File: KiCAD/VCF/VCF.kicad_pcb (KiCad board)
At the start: 2 copper layers, 50 x 100 mm, 50 parts, among them J1 FM, J2 CV, J3 IN, J4 OUT, J5 Conn_01x03, J6 Conn_01x03, Q1 2N3904, SW1 SW_SPDT, SW2 SW_SPDT, U1 TL072, U2 TL072, U3 UA776, U4 UA776, U5 TL072

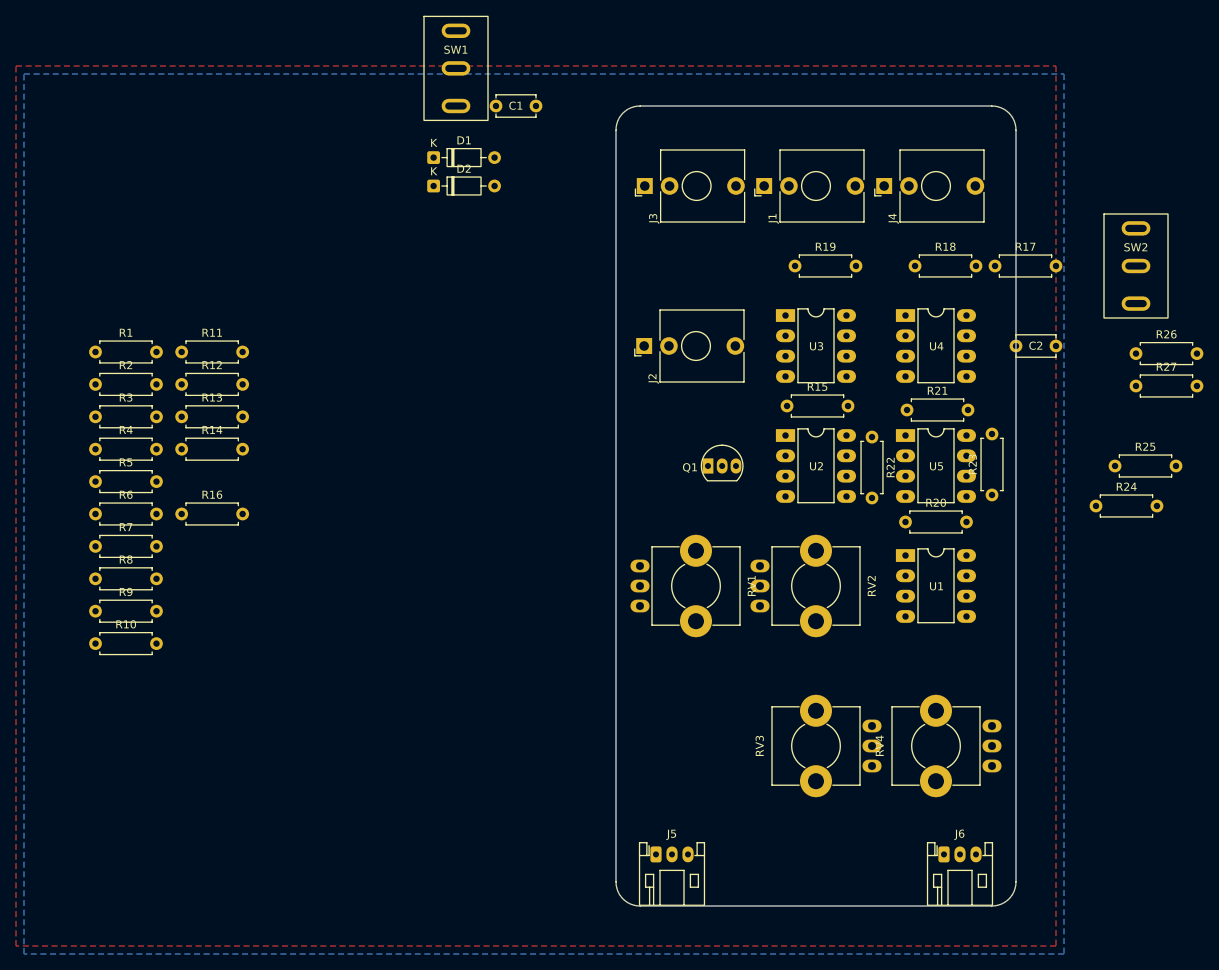
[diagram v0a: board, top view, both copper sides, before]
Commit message: VCF PCB
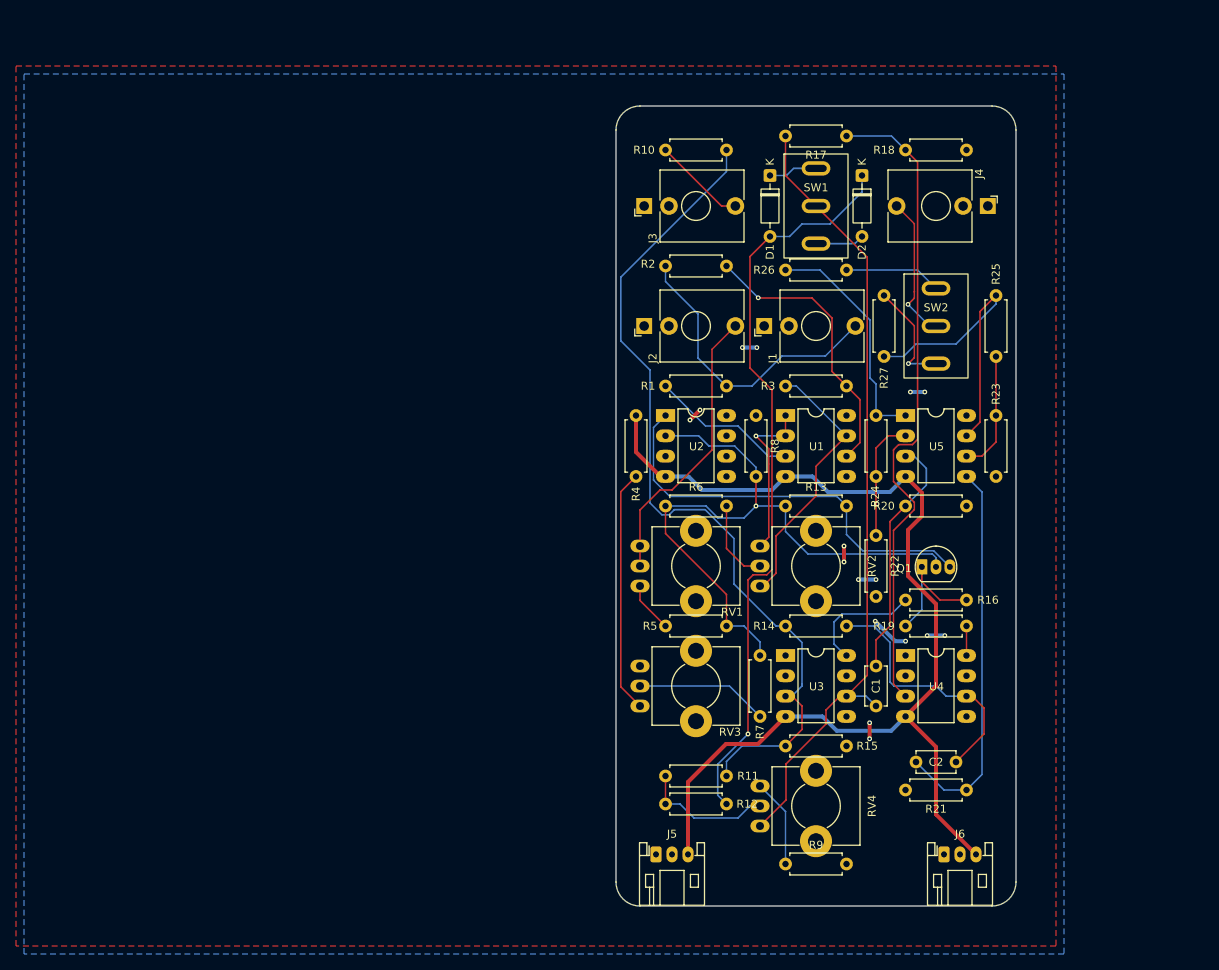
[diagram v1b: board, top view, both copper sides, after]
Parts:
- added Ref**: Val**, HackSynth:PancakeLegend Logo - 10mm, B.Cu at (194.5, 77.8)
- added Ref**: Val**, HackSynth:CCHS Logo - 10mm, B.Cu at (194.0, 62.2)
- moved R10 100.1 mm to (138.8, 55.5), turned to 180 degrees
- moved R16 98.7 mm to (168.8, 111.8), turned to 180 degrees
- moved R9 91.9 mm to (146.2, 144.8)
- moved C1 88.8 mm to (157.5, 125.0), turned to 90 degrees
- moved R3 86.3 mm to (146.2, 85.0)
- moved R11 86.3 mm to (138.8, 133.8), turned to 180 degrees
- moved R14 86.0 mm to (153.8, 115.0), turned to 180 degrees
- moved R12 86.0 mm to (138.8, 137.2), turned to 180 degrees
- moved R8 85.0 mm to (142.5, 88.7), turned to -90 degrees
- moved R7 84.2 mm to (143.0, 118.7), turned to -90 degrees
- moved R5 80.9 mm to (138.8, 115.0), turned to 180 degrees
- moved R2 80.2 mm to (138.8, 70.0), turned to 180 degrees
- moved R13 76.3 mm to (146.2, 100.0)
- moved R1 71.4 mm to (131.2, 85.0)
- moved R6 71.3 mm to (131.2, 100.0)
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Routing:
- net VSS: track 0.00 -> 139.1 mm
- net Net-(U3-+): track 0.00 -> 107.6 mm
- net Net-(SW1-B): track 0.00 -> 100.7 mm
- net Net-(D1-A): track 0.00 -> 93.2 mm, vias 0 -> 1
- net Net-(Q1-B): track 0.00 -> 83.4 mm, vias 0 -> 1
- net Net-(U4-+): track 0.00 -> 82.0 mm
- net Net-(Q1-E): track 0.00 -> 52.5 mm
- net Net-(U5B-+): track 0.00 -> 48.6 mm
- net Net-(J1-PadT): track 0.00 -> 37.4 mm
- net Net-(R25-Pad1): track 0.00 -> 36.8 mm
- net Net-(J2-PadT): track 0.00 -> 35.8 mm
- net Net-(U1B--): track 0.00 -> 35.3 mm, vias 0 -> 1
- net Net-(R3-Pad1): track 0.00 -> 33.7 mm
- net Net-(C2-Pad1): track 0.00 -> 32.5 mm
- net Net-(U5A-+): track 0.00 -> 30.6 mm
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- added copper zone on B.Cu, net VDD
- removed copper zone on B.Cu, net GND
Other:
- board text added: "PancakeLegend 2025"
- board text added: "VCF v1-0"
